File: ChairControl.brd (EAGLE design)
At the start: 150 x 84 mm, 22 parts, among them J1 Digital_0_7, J2 Analog, J3 Digital_8_13, SW1 TL46WO, X1 INPUT, X2 OUTPUT, X4 INPUT

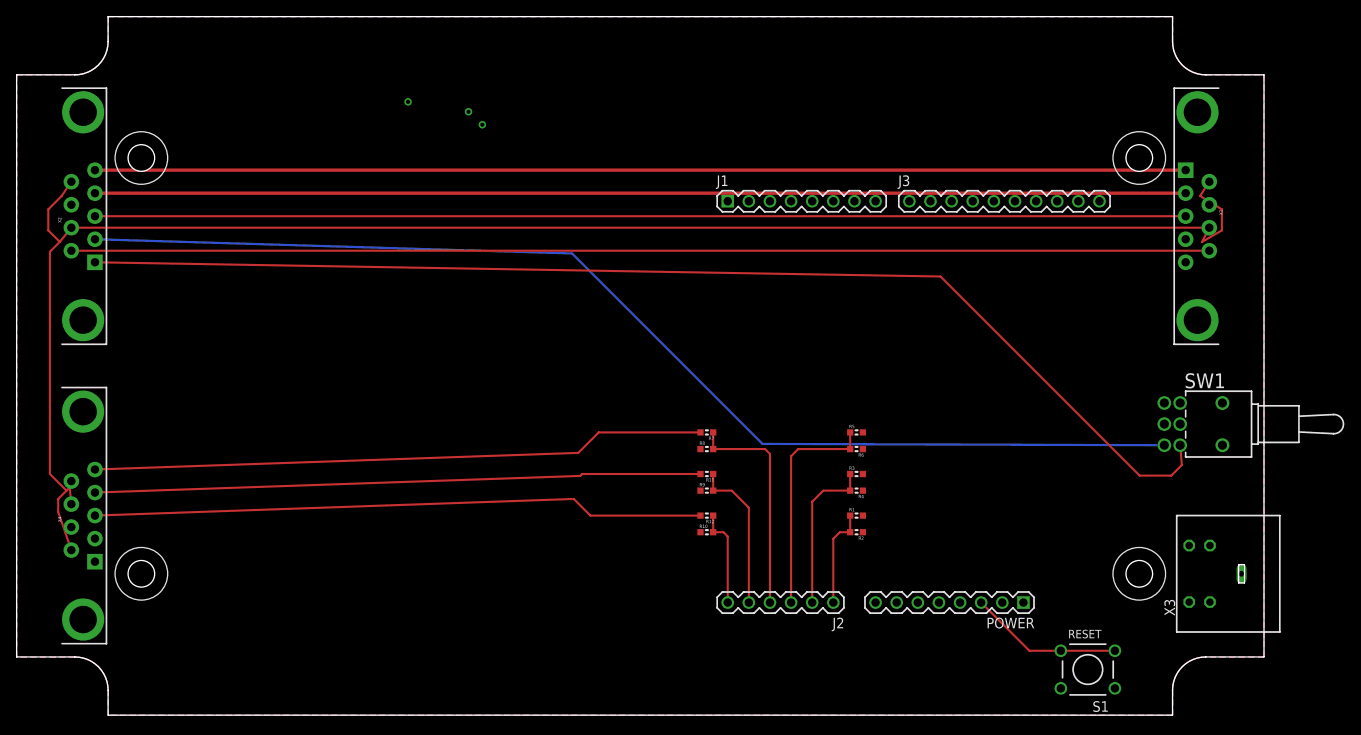
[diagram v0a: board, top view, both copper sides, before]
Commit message: Routing and silkscreen
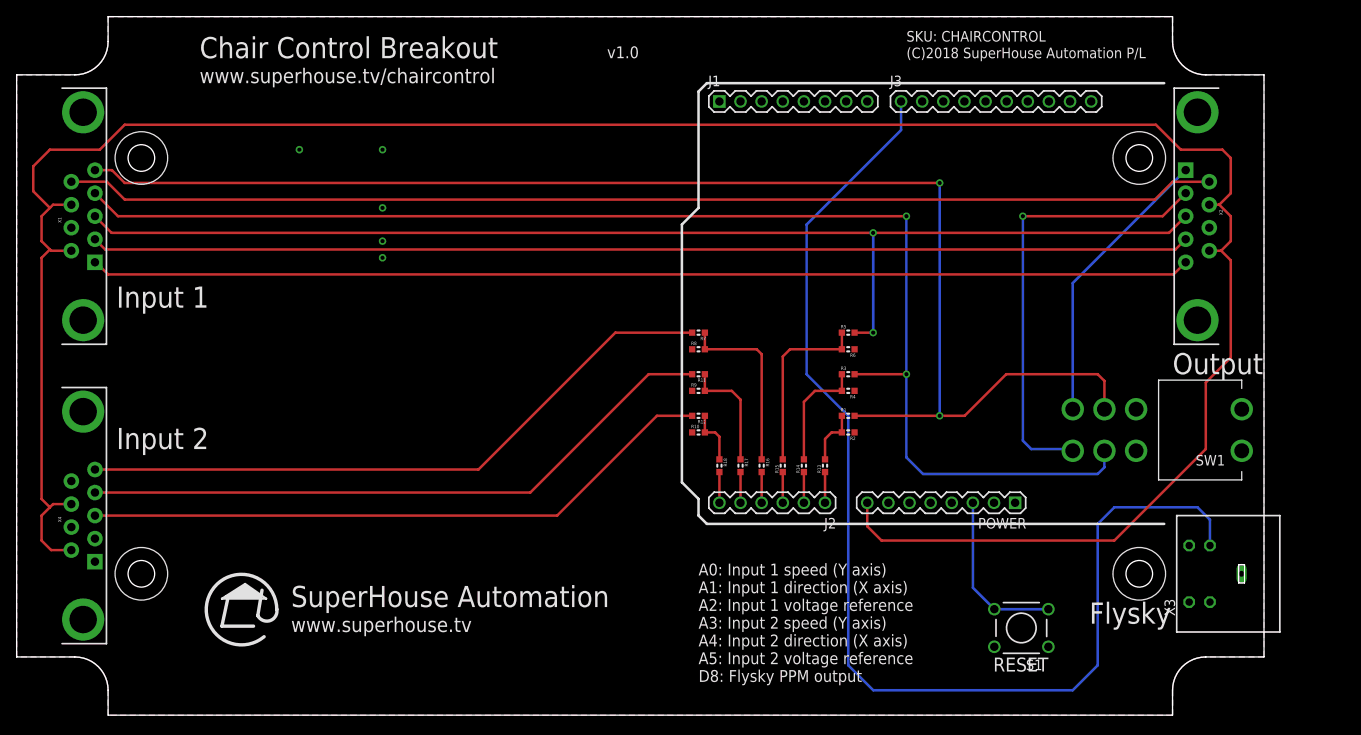
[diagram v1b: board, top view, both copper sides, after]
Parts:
- added R13, R14, R15, R16, R17, R18: 1K, freetronics-jon:0603
- SW1: value TL46WO -> SWITCH-DPDT3; device switch:TL4XWO -> freetronics-jon:7201SD9AV2BE
- moved X1 134.0 mm to (8.00, 60.0), turned to 90 degrees
- moved X2 134.0 mm to (142.0, 60.0), turned to 270 degrees
- moved J1 12.0 mm to (84.5, 73.8)
- moved J2 12.0 mm to (97.2, 25.5)
- moved J3 12.0 mm to (106.4, 73.8)
- moved POWER 12.0 mm to (120.1, 25.5)
- moved R1 12.0 mm to (100.0, 36.0)
- moved R10 12.0 mm to (82.0, 34.0)
- moved R11 12.0 mm to (82.0, 41.0)
- moved R12 12.0 mm to (82.0, 36.0)
- moved R2 12.0 mm to (100.0, 34.0)
- moved R3 12.0 mm to (100.0, 41.0)
- moved R4 12.0 mm to (100.0, 39.0)
- moved R5 12.0 mm to (100.0, 46.0)
- moved R6 12.0 mm to (100.0, 44.0)
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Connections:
- new net N$2: R1.1, R13.2, R2.2
- new net N$3: R14.2, R3.1, R4.2
- new net N$4: R15.2, R5.1, R6.2
- new net N$7: R16.1, R7.1, R8.2
- new net N$8: R11.1, R17.1, R9.2
- new net N$9: R10.2, R12.1, R18.1
- net A0: now also R13.1; no longer R1.1, R2.2
- net A1: now also R14.1; no longer R3.1, R4.2
- net A2: now also R15.1; no longer R5.1, R6.2
- net A3: now also R16.2; no longer R7.1, R8.2
- net A4: now also R17.2; no longer R11.1, R9.2
- net A5: now also R18.2; no longer R10.2, R12.1
- net DIRECTION_OUT: now also SW1.4; no longer SW1.6
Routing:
- net SPEED_IN: track 0.00 -> 166.1 mm, vias 0 -> 2
- net DIRECTION_IN: track 0.00 -> 160.9 mm, vias 0 -> 2
- net D8: track 0.00 -> 142.1 mm
- net SPEED_OUT: track 143.5 -> 34.4 mm
- net 12V: track 201.8 -> 297.6 mm
- net DIRECTION_OUT: track 138.1 -> 54.2 mm, vias 0 -> 1
- net A2: track 27.1 -> 3.70 mm
- net A3: track 26.9 -> 3.70 mm
- net N$4: track 0.00 -> 21.8 mm
- net N$7: track 0.00 -> 21.7 mm
- net REFERENCE: track 131.2 -> 147.1 mm, vias 0 -> 2
- net A1: track 19.2 -> 3.70 mm
- net A4: track 18.5 -> 3.70 mm
- net N$3: track 0.00 -> 14.0 mm
- net N$8: track 0.00 -> 13.9 mm
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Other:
- board text added: "(C)2018 SuperHouse Automation P/L"
- board text added: "A0: Input 1 speed (Y axis) A1: Input 1 direction (X axis) A2: Input 1 voltage reference A3: Input 2 speed (Y axis) A4: Input 2 direction (X axis) A5: Input 2 voltage reference D8: Flysky PPM output"
- board text added: "Chair Control Breakout"
- board text added: "Flysky"
- board text added: "Input 1"
- board text added: "Input 2"
- board text added: "Output"
- board text added: "SKU: CHAIRCONTROL"
- board text added: "SuperHouse Automation"
- board text added: "v1.0"
- board text added: "www.superhouse.tv"
- board text added: "www.superhouse.tv/chaircontrol"
